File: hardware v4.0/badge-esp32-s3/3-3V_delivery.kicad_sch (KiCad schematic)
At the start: 27 parts, among them Q4 HL2301A, Q7 AO3424, U2 TPS630701RNMR, U9 AP63203WU-7

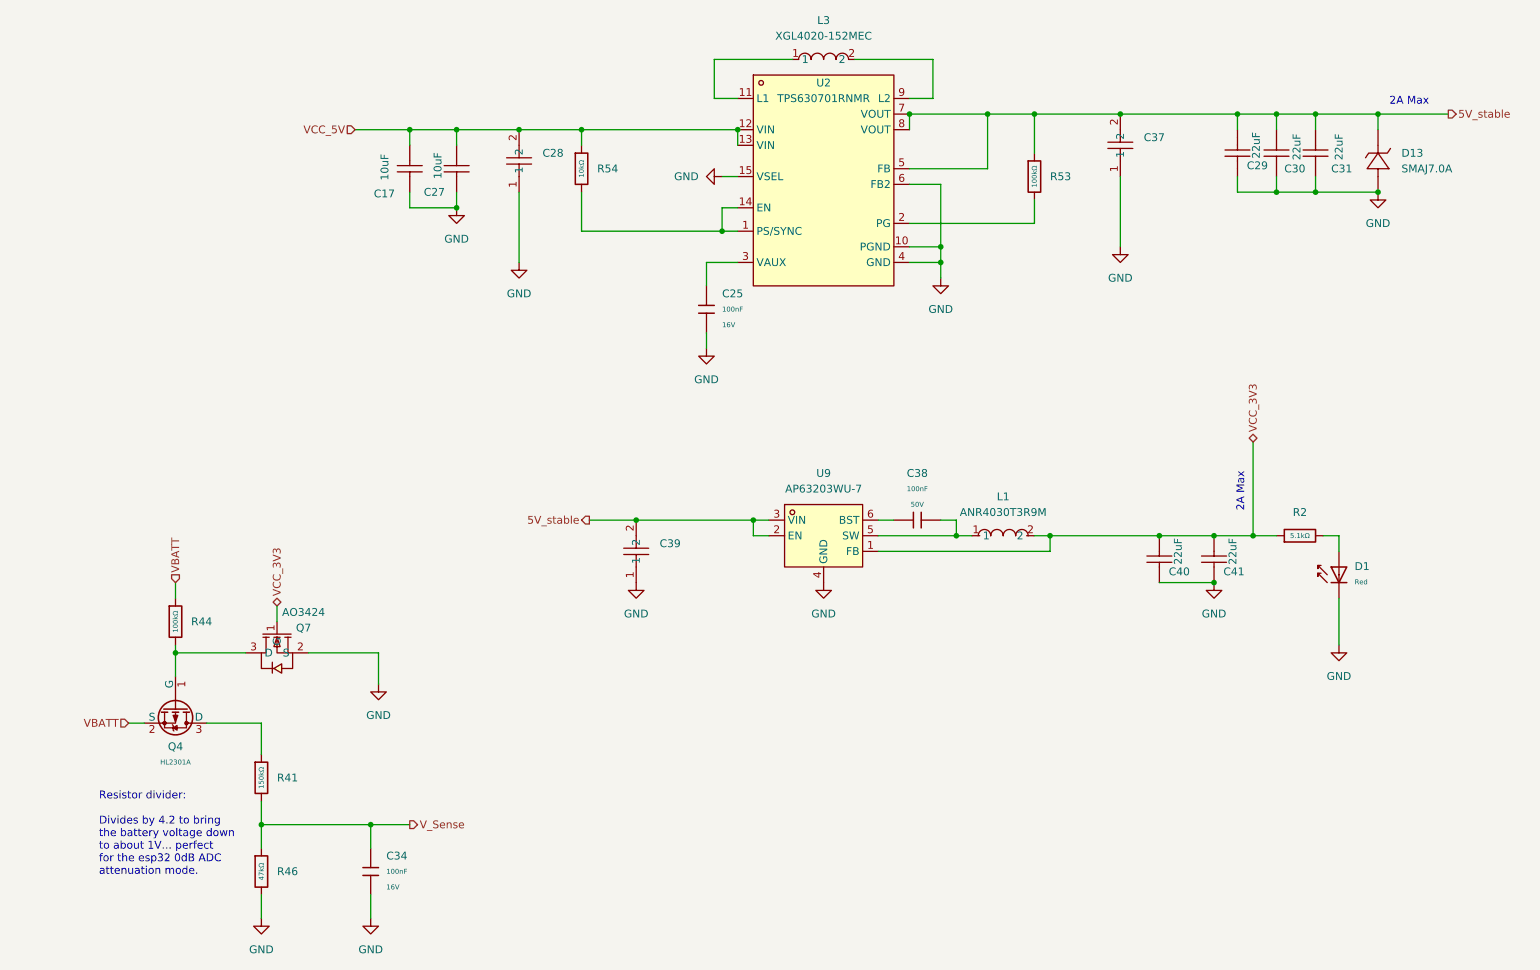
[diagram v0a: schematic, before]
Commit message: finished schematics and layout
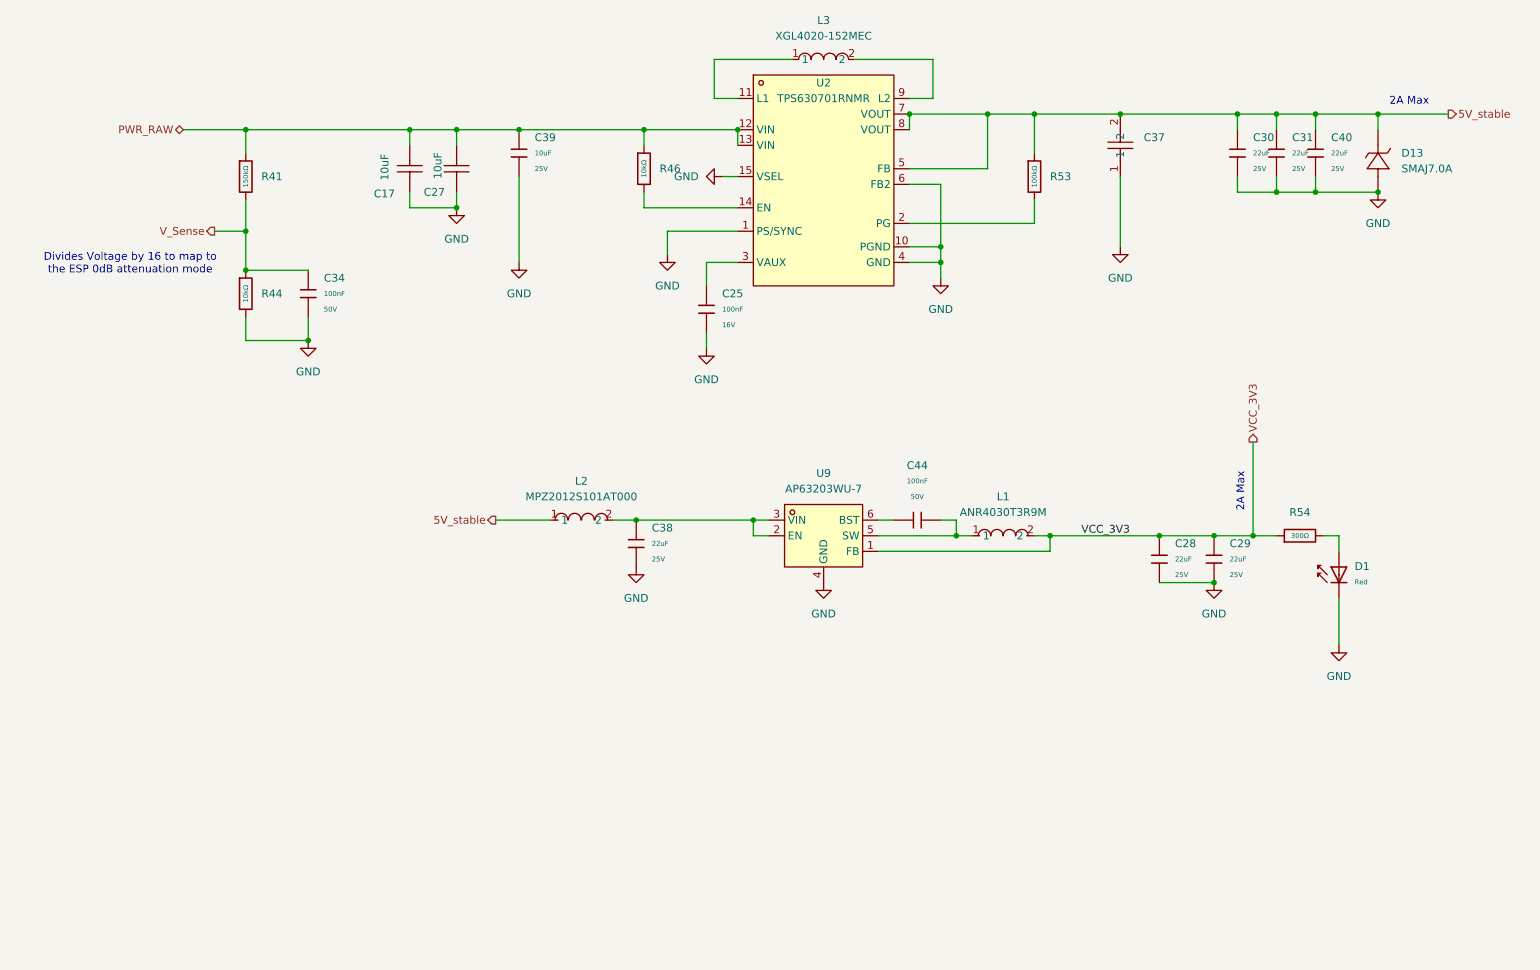
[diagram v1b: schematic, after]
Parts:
- removed C28, C39: TMK107BBJ106MA-T, lcsc-lib:C0603, symbol lcsc-lib:TMK107BBJ106MA-T
- removed C29, C30, C31, C40, C41: 22uF, lcsc-lib:C0805, symbol lcsc-lib:EMK212BBJ226MG-T
- removed C34: 100nF, PCM_JLCPCB:C_0402, symbol PCM_JLCPCB-Capacitors:0402,100nF
- removed C38: 100nF, PCM_JLCPCB:C_0603, symbol PCM_JLCPCB-Capacitors:0603,100nF
- removed Q4: HL2301A, PCM_JLCPCB:Q_SOT-23, symbol PCM_JLCPCB-Transistors:PMOS,HL2301A
- removed Q7: AO3424, lcsc-lib:SC-59-3_L2.9-W1.6-P0.95-LS2.9-BR, symbol lcsc-lib:AO3424
- removed R2: 5.1kΩ, PCM_JLCPCB:R_0402, symbol PCM_JLCPCB-Resistors:0402,5.1kΩ
- removed R44: 100kΩ, PCM_JLCPCB:R_0402, symbol PCM_JLCPCB-Resistors:0402,100kΩ
- removed R46: 47kΩ, PCM_JLCPCB:R_0402, symbol PCM_JLCPCB-Resistors:0402,47kΩ
- removed R54: 10kΩ, PCM_JLCPCB:R_0402, symbol PCM_JLCPCB-Resistors:0402,10kΩ
- added C28, C29, C30, C31, C38, C40: 22uF, PCM_JLCPCB:C_0805, symbol PCM_JLCPCB-Capacitors:0805,22uF
- added C34, C44: 100nF, PCM_JLCPCB:C_0402, symbol PCM_JLCPCB-Capacitors:0402,100nF,(2)
- added C39: 10uF, PCM_JLCPCB:C_0603, symbol PCM_JLCPCB-Capacitors:0603,10uF,(2)
- added L2: MPZ2012S101AT000, lcsc-lib:L0805, symbol lcsc-lib:MPZ2012S101AT000
- added R44, R46: 10kΩ, PCM_JLCPCB:R_0402, symbol PCM_JLCPCB-Resistors:0402,10kΩ
- added R54: 300Ω, PCM_JLCPCB:R_0402, symbol PCM_JLCPCB-Resistors:0402,300Ω
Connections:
- net VCC_5V is gone; now on net PWR_RAW: C17.2, C27.2, U2.12 (VIN), U2.13 (VIN)
- net 5V_stable: now also C30.1, C31.1, C40.1, L2.1; no longer U9.2 (EN), U9.3 (VIN)
- net GND: now also U2.1 (PS/SYNC), C28.2, C29.2, C30.2, C31.2, C34.2, C38.2, C39.2, C40.2, R44.2
- net VCC_3V3: now also C28.1, C29.1, R54.1
- net V_Sense: now also C34.1, R44.1
- net at D1.2: now also R54.2
- net PWR_RAW: now reaches R41.1
- net PWR_RAW: now also C39.1, R46.1
- net at L1.1, U9.5 (SW): now also C44.2
- net at U2.14 (EN): now also R46.2; no longer U2.1 (PS/SYNC)
- net at U9.6 (BST): now also C44.1
- new net: C38.1, L2.2, U9.2 (EN), U9.3 (VIN)
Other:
- note added: "Divides Voltage by 16 to map to the ESP 0dB attenuation mode"
- note removed: "Resistor divider: Divides by 4.2 to bring the battery voltage down to about 1V... perfect for the esp32 0dB ADC attenuation mode."
